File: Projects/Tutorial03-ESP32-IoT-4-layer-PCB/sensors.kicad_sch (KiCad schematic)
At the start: 18 parts, among them Q1 TEMT6000X01, U2 MAX4466EXK, U7 BME280

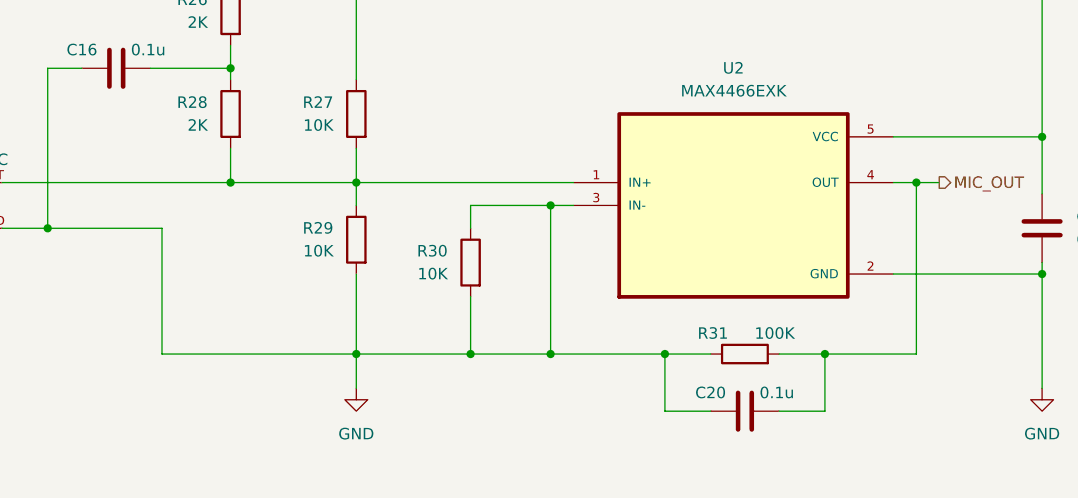
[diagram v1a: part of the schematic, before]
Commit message: 20260513
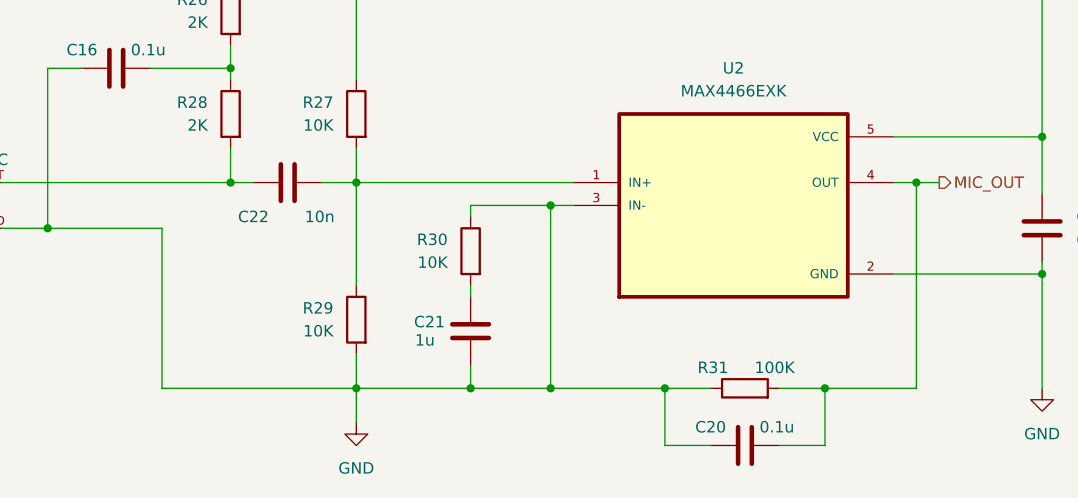
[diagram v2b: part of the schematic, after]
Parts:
- added C21: 1u, Capacitor_SMD:C_0805_2012Metric, symbol Device:C
- added C22: 10n, Capacitor_SMD:C_0805_2012Metric, symbol Device:C
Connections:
- net GND: now also C21.2; no longer R30.2
- net at R27.2, R29.1, U2.1 (IN+): now also C22.2; no longer MK1.OUT, R28.2
- new net: C21.1, R30.2
- new net: C22.1, MK1.OUT, R28.2
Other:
- moved on the sheet: C20, R29, R30, R31
